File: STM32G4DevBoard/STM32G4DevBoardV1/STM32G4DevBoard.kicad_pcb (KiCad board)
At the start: 4 copper layers, 44.7 x 23.5 mm, 26 parts, among them J1 USB_B_Micro, J2 Conn_01x13, J3 Conn_01x13, U1 STM32G431KBTx, U2 LD3985M33R_SOT23, Y1 24MHz

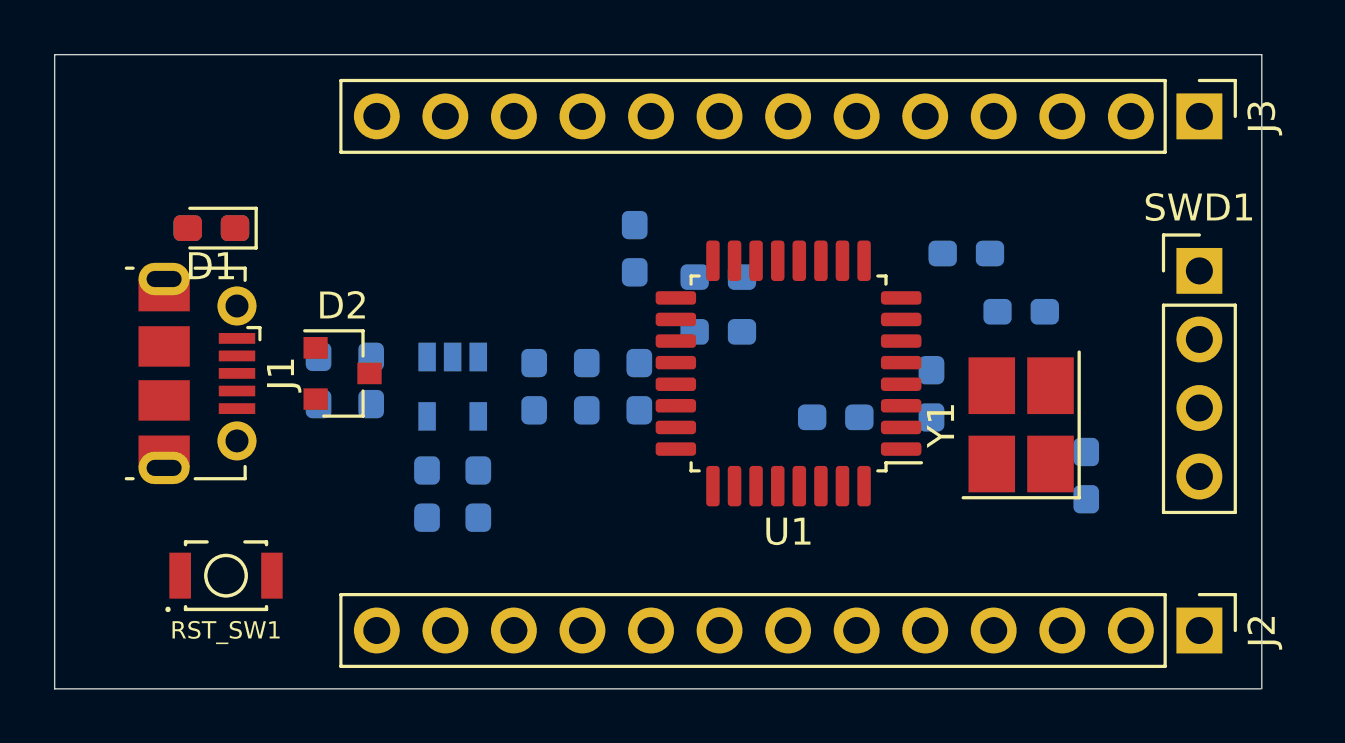
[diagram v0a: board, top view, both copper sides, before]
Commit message: Finished Crystal Layout
Made changes for crystal layout
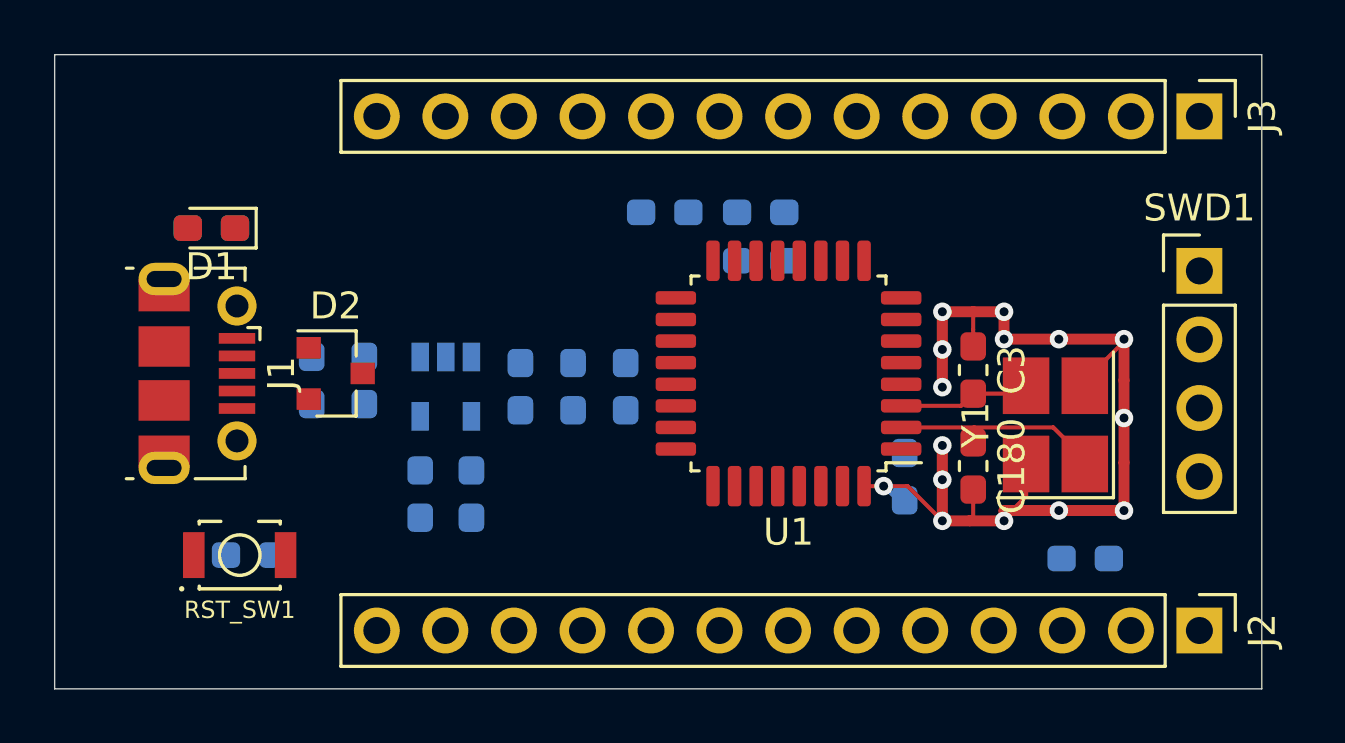
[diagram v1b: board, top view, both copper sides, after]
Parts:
- C180, C3: moved to F.Cu
- moved C1 31.1 mm to (112.4, 98.0), turned to 180 degrees
- moved R1 10.6 mm to (143.3, 98.2), turned to 180 degrees
- moved C180 5.99 mm to (139.2, 94.7), turned to 270 degrees
- moved C3 4.33 mm to (139.2, 91.2), turned to 270 degrees
- moved C7 3.23 mm to (136.7, 95.1)
- moved C4 3.07 mm to (131.3, 87.1)
- moved C5 2.87 mm to (131.3, 85.3)
- moved FB1 1.75 mm to (127.8, 85.3), turned to 0 degrees
- moved Y1 1.27 mm to (142.2, 93.2)
- moved RST_SW1 0.92 mm to (112.0, 98.0)
- moved C11 0.51 mm to (122.4, 91.8)
- moved C6 0.51 mm to (124.4, 91.8)
- moved C8 0.51 mm to (126.3, 91.8)
- moved C10 0.25 mm to (116.6, 91.6)
- moved C12 0.25 mm to (118.7, 95.8)
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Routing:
- net GND: track 0.00 -> 38.3 mm, vias 0 -> 15
- net OSC_IN: track 0.00 -> 8.04 mm
- net OSC_OUT: track 0.00 -> 4.94 mm
